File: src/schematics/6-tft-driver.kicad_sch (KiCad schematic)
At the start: 39 parts, among them Q601 NX6008NBKW, Q602 BC847BS, Q603 BC847BS, U601 TMUX1574RSV, U602 TMUX1574RSV, U603 TMUX1574RSV

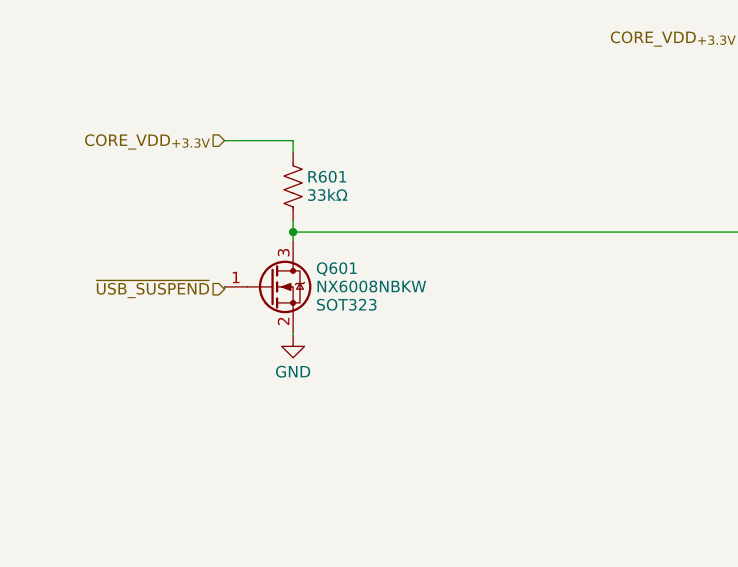
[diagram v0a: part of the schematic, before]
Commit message: PCB routing.
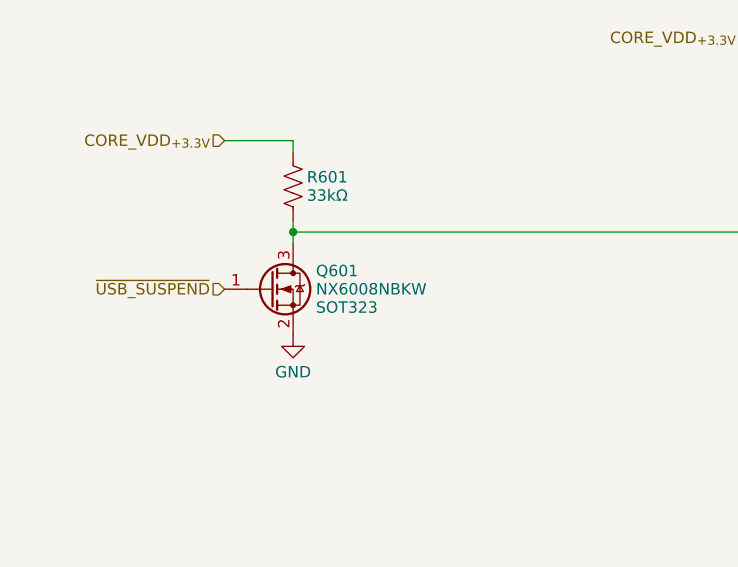
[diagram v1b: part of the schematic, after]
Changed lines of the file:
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@@
     (stroke (width 0) (type default))
   )
-  (wire (pts (xy 60.96 52.07) (xy 60.96 53.086))
+  (wire (pts (xy 60.96 52.07) (xy 60.96 53.34))
     (stroke (width 0) (type default))
   )
@@
     (stroke (width 0) (type default))
   )
-  (wire (pts (xy 60.96 63.246) (xy 60.96 63.5))
-    (stroke (width 0) (type default))
-  )
   (bus (pts (xy 88.9 223.52) (xy 88.9 231.14))
     (stroke (width 0) (type default))
@@
   )
   (wire (pts (xy 327.66 73.66) (xy 360.68 73.66))
-    (stroke (width 0) (type default))
-  )
-  (wire (pts (xy 53.34 58.166) (xy 53.34 58.42))
     (stroke (width 0) (type default))
   )
@@
     )
   )
-  (symbol (lib_id "restall-manufacturer-nexperia:NX6008NBKW") (at 58.42 58.166 0) (unit 1)
+  (symbol (lib_id "restall-manufacturer-nexperia:NX6008NBKW") (at 58.42 58.42 0) (unit 1)
     (in_bom yes) (on_board yes) (dnp no)
-    (property "Reference" "Q601" (at 63.5 56.134 0)
-      (effects (font (size 1.27 1.27)) (justify left))
-    )
-    (property "Value" "NX6008NBKW" (at 63.5 58.166 0)
-      (effects (font (size 1.27 1.27)) (justify left))
-    )
-    (property "Footprint" "restall-generic-sot:SOT323" (at 63.5 54.61 0)
-      (effects (font (size 1.27 1.27)) (justify left) hide)
-    )
-    (property "Datasheet" "https://assets.nexperia.com/documents/data-sheet/NX6008NBKW.pdf" (at 63.5 66.294 0)
-      (effects (font (size 1.27 1.27)) (justify left) hide)
-    )
-    (property "Package" "SOT323" (at 63.5 60.198 0)
-      (effects (font (size 1.27 1.27)) (justify left))
-    )
-    (property "Manufacturer" "Nexperia" (at 63.5 64.008 0)
-      (effects (font (size 1.27 1.27)) (justify left) hide)
-    )
-    (property "ManufacturerPartNumber" "NX6008NBKW" (at 63.5 61.722 0)
-      (effects (font (size 1.27 1.27)) (justify left) hide)
-    )
+    (property "Reference" "Q601" (at 63.5 56.388 0)
+      (effects (font (size 1.27 1.27)) (justify left))
+    )
+    (property "Value" "NX6008NBKW" (at 63.5 58.42 0)
+      (effects (font (size 1.27 1.27)) (justify left))
+    )
+    (property "Footprint" "restall-generic-sot:SOT323" (at 63.5 54.864 0)
+      (effects (font (size 1.27 1.27)) (justify left) hide)
+    )
+    (property "Datasheet" "https://assets.nexperia.com/documents/data-sheet/NX6008NBKW.pdf" (at 63.5 66.548 0)
+      (effects (font (size 1.27 1.27)) (justify left) hide)
+    )
+    (property "Package" "SOT323" (at 63.5 60.452 0)
+      (effects (font (size 1.27 1.27)) (justify left))
+    )
+    (property "Manufacturer" "Nexperia" (at 63.5 64.262 0)
+      (effects (font (size 1.27 1.27)) (justify left) hide)
+    )
+    (property "ManufacturerPartNumber" "NX6008NBKW" (at 63.5 61.976 0)
+      (effects (font (size 1.27 1.27)) (justify left) hide)
+    )
